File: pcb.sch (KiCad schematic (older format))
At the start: 76 parts, among them SW1 SW_Push, U1 ATmega32U4-AU, Y1 16MHz

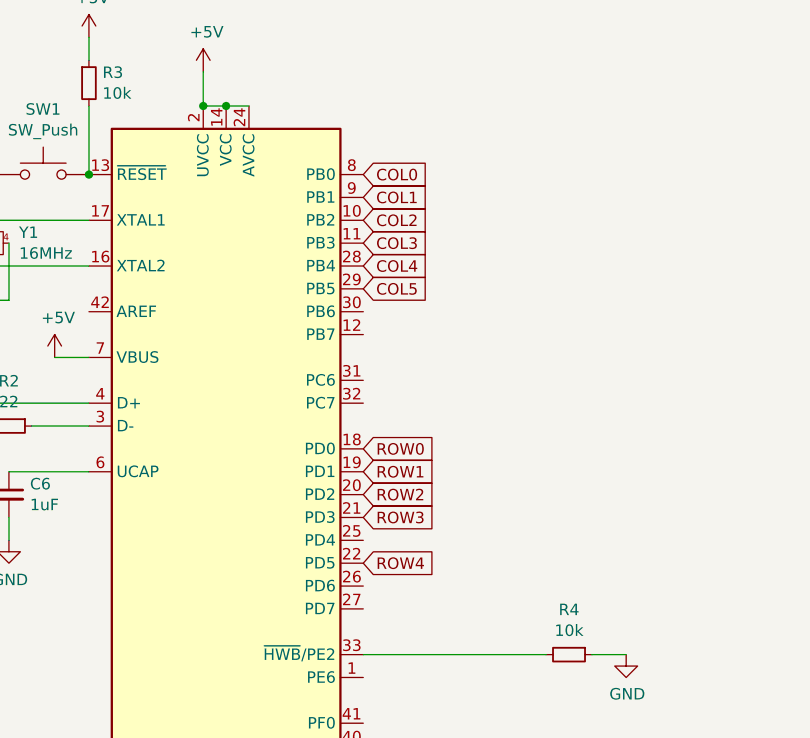
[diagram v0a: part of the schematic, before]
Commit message: Moved Things Around
Still not sure this is any good
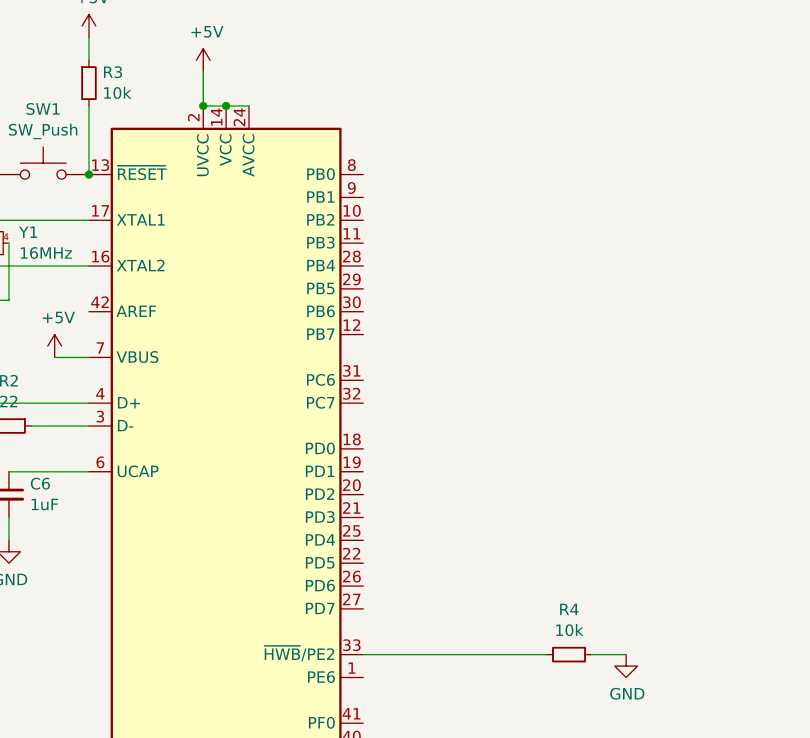
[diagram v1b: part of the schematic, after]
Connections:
- net COL0: no longer U1.8 (PB0)
- net COL1: no longer U1.9 (PB1)
- net COL2: no longer U1.10 (PB2)
- net COL3: no longer U1.11 (PB3)
- net COL4: no longer U1.28 (PB4)
- net COL5: no longer U1.29 (PB5)
- net ROW0: no longer U1.18 (PD0)
- net ROW1: no longer U1.19 (PD1)
- net ROW2: no longer U1.20 (PD2)
- net ROW3: no longer U1.21 (PD3)
- net ROW4: no longer U1.22 (PD5)
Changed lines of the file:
@@
 Text GLabel 7000 5250 0    50   Input ~ 0
 ROW4
-Text GLabel 3600 2400 2    50   Input ~ 0
-COL0
-Text GLabel 3600 2500 2    50   Input ~ 0
-COL1
-Text GLabel 3600 2600 2    50   Input ~ 0
-COL2
-Text GLabel 3600 2700 2    50   Input ~ 0
-COL3
-Text GLabel 3600 2800 2    50   Input ~ 0
-COL4
-Text GLabel 3600 2900 2    50   Input ~ 0
-COL5
-Text GLabel 3600 3600 2    50   Input ~ 0
-ROW0
-Text GLabel 3600 3700 2    50   Input ~ 0
-ROW1
-Text GLabel 3600 3800 2    50   Input ~ 0
-ROW2
-Text GLabel 3600 3900 2    50   Input ~ 0
-ROW3
-Text GLabel 3600 4100 2    50   Input ~ 0
-ROW4
 $EndSCHEMATC
